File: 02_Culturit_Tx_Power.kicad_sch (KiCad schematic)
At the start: 36 parts, among them U10 TPS22916CNYFPT, U11 SN74AUP2G08RSER, U12 TPS22916CNYFPT, U5 TPS3839A09DBZR, U6 TPS22916CNYFPT, U7 LP5907QMFX-2.8Q1, U8 TPS6282618DMQR, U9 SN74AUP2G08RSER

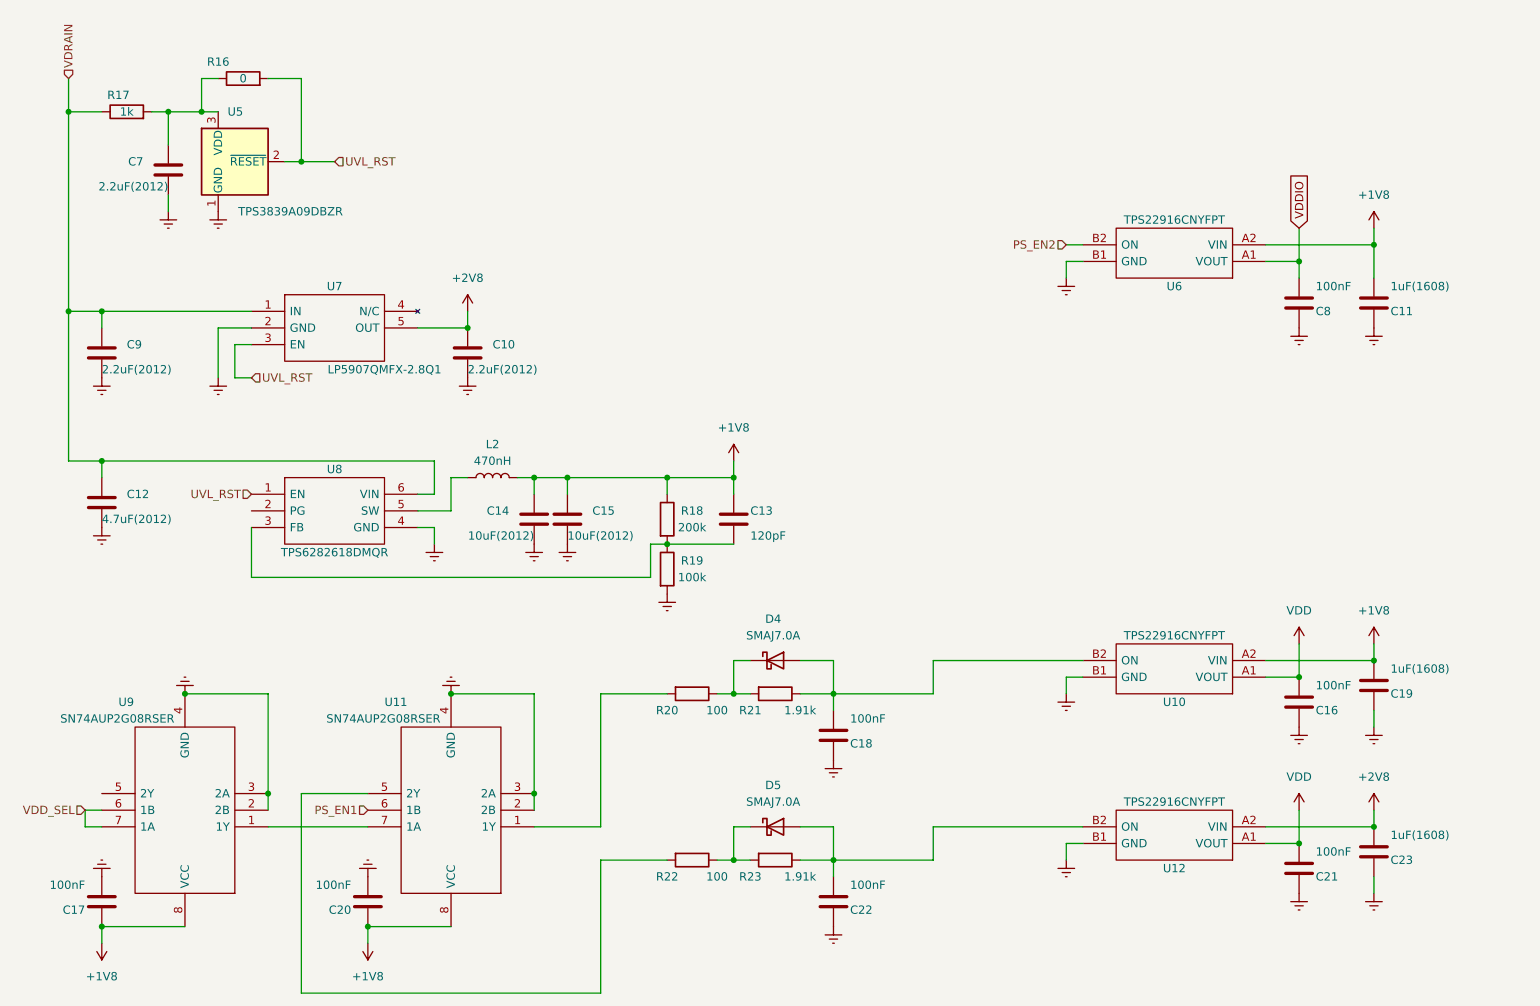
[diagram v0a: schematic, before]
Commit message: 2022-08-26
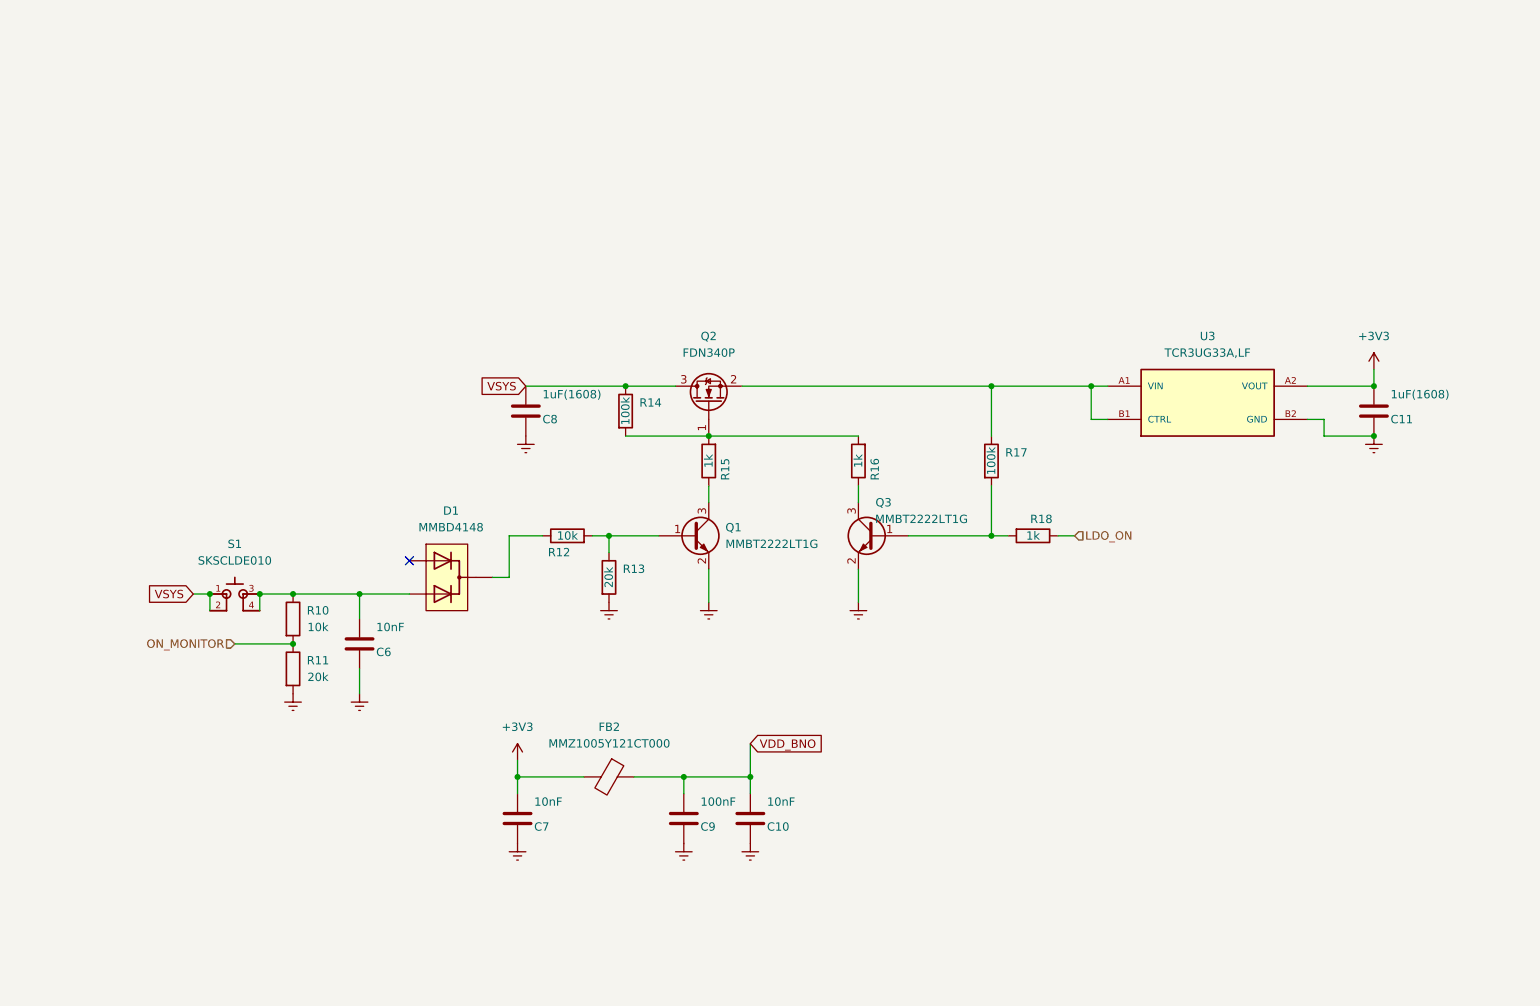
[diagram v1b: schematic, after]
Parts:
- removed C12: 4.7uF(2012), Capacitor_SMD:C_0805_2012Metric, symbol Device:C
- removed C13: 120pF, Capacitor_SMD:C_0402_1005Metric, symbol Device:C
- removed C14, C15: 10uF(2012), Capacitor_SMD:C_0805_2012Metric, symbol Device:C
- removed C16, C17, C18, C20, C21, C22, C8: 100nF, Capacitor_SMD:C_0402_1005Metric, symbol Device:C
- removed C19, C23: 1uF(1608), Capacitor_SMD:C_0603_1608Metric, symbol Device:C
- removed D4, D5: SMAJ7.0A, Diode_SMD:D_SMA, symbol Device:D_Schottky
- removed L2: 470nH, Inductor_SMD:L_0805_2012Metric, symbol Device:L
- removed R20, R22: 100, Resistor_SMD:R_0402_1005Metric, symbol Device:R
- removed R21, R23: 1.91k, Resistor_SMD:R_0402_1005Metric, symbol Device:R
- removed U10, U12, U6: TPS22916CNYFPT, Local_devices:BGA4C40P2X2_78X78X50, symbol TPS22916CNYFPT:TPS22916CNYFPT
- removed U11, U9: SN74AUP2G08RSER, Local_devices:RSE0008A, symbol SN74AUP2G08RSER:SN74AUP2G08RSER
- removed U5: TPS3839A09DBZR, Package_TO_SOT_SMD:SOT-23, symbol Power_Supervisor:TPS3839DBZ
- removed U7: LP5907QMFX-2.8Q1, Local_devices:SOT95P280X145-5N, symbol LP5907QMFX-2.8Q1:LP5907QMFX-2.8Q1
- removed U8: TPS6282618DMQR, Local_devices:TPS6282618DMQR, symbol TPS6282618DMQR:TPS6282618DMQR
- added C11: 1uF(1608), Capacitor_SMD:C_0603_1608Metric, symbol Device:C
- added C6: 10nF, Capacitor_SMD:C_0402_1005Metric, symbol Device:C
- added D1: MMBD4148, Local_devices:SOT23, symbol MMBD4148:MMBD4148
- added FB2: MMZ1005Y121CT000, symbol Device:FerriteBead
- added Q1, Q3: MMBT2222LT1G, Local_devices:SOT23, symbol Device:Q_NPN_BEC
- added Q2: FDN340P, Local_devices:SOT23, symbol Device:Q_NMOS_GSD
- added R10, R12: 10k, Resistor_SMD:R_0402_1005Metric, symbol Device:R
- added R11, R13: 20k, Resistor_SMD:R_0402_1005Metric, symbol Device:R
- added R15: 1k, Resistor_SMD:R_0402_1005Metric, symbol Device:R
- added S1: SKSCLDE010, Local_devices:SKSCLDE010, symbol SKSCLDE010:SKSCLDE010
- added U3: TCR3UG33A,LF, Local_devices:BGA4N35P2X2_64X64X33, symbol TCR3UG33A_LF:TCR3UG33A,LF
- C10, C7: value 2.2uF(2012) -> 10nF; footprint Capacitor_SMD:C_0805_2012Metric -> Capacitor_SMD:C_0402_1005Metric; MPN CC0805KKX7R8BB225 -> CC0402KRX7R9BB103
- C9: value 2.2uF(2012) -> 100nF; footprint Capacitor_SMD:C_0805_2012Metric -> Capacitor_SMD:C_0402_1005Metric; MPN CC0805KKX7R8BB225 -> CC0402KRX7R7BB104
- R16: value 0 -> 1k; MPN 0402WGF0000TCE -> RC0402FR-071KL
- R17: value 1k -> 100k; MPN 0402WGJ0102TCE -> RC0402FR-07100KL
- R18: value 200k -> 1k; MPN RTT022003FTH -> RC0402FR-071KL
- renumbered C11 to C8, R19 to R14
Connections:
- net +2V8 is gone; now on net Earth: C10.2
- net Earth: now also C7.2, C9.2, C11.2, C6.2, Q1.2 (E), Q3.2 (E), R11.2, R13.2, U3.B2 (GND); no longer C10.1, C7.1, C9.1, R14.2
- net at R18.2: now also R17.2, Q3.1 (B); no longer R14.1
- net +1V8 renamed LDO_ON
- net LDO_ON: no longer C8.1
- net UVL_RST: no longer names the net of R16.2
- net UVL_RST: now also R14.2, Q2.1 (G), R15.2
- net VDRAIN: no longer names the net of R17.1
- net VDRAIN: now also Q2.2 (S), U3.A1 (VIN), U3.B1 (CTRL); no longer C9.2
- new net: Q3.3 (C), R16.1
- new net: C6.1, D1.2, R10.1, S1.3, S1.4
- new net: Q1.1 (B), R12.2, R13.1
- new net: Q1.3 (C), R15.1
- new net: D1.3, R12.1
- new net +3V3: C11.1, C7.1, FB2.2, U3.A2 (VOUT)
- new net ON_MONITOR: R10.2, R11.1
- new net VDD_BNO: C10.1, C9.1, FB2.1
- new net VSYS: C8.1, Q2.3 (D), R14.1, S1.1, S1.2
- no-connect marks 0 -> 1
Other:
- moved on the sheet: C8, R14

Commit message: 2022-08-29
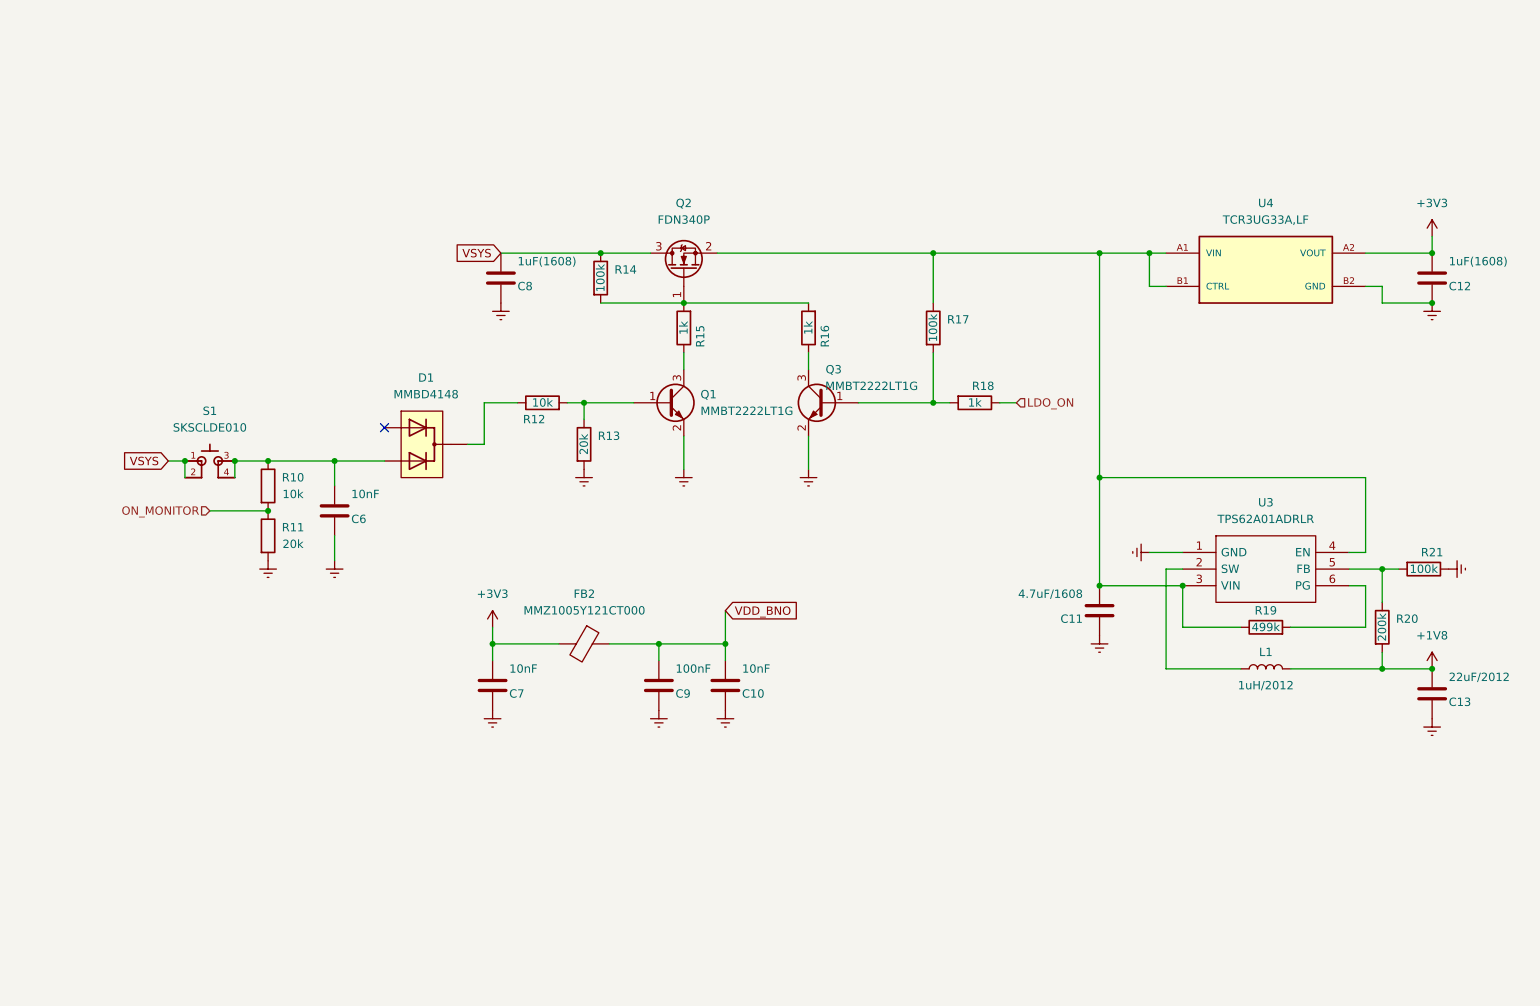
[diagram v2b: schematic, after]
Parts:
- added C11: 4.7uF/1608, Capacitor_SMD:C_0603_1608Metric, symbol Device:C
- added C13: 22uF/2012, Capacitor_SMD:C_0805_2012Metric, symbol Device:C
- added L1: 1uH/2012, Inductor_SMD:L_0805_2012Metric, symbol Device:L
- added R19: 499k, Resistor_SMD:R_0402_1005Metric, symbol Device:R
- added R20: 200k, Resistor_SMD:R_0402_1005Metric, symbol Device:R
- added R21: 100k, Resistor_SMD:R_0402_1005Metric, symbol Device:R
- added U3: TPS62A01ADRLR, Local_devices:SOTFL50P160X60-6N, symbol TPS62A01ADRLR:TPS62A01ADRLR
- renumbered C11 to C12, U3 to U4
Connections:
- net Earth: now also C11.2, C13.2, R21.1, U3.1 (GND)
- net at Q2.2 (S), R17.1, U4.A1 (VIN)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: now also C11.1, R19.1, U3.3 (VIN), U3.4 (EN)
- new net: L1.1, U3.2 (SW)
- new net: R20.1, R21.2, U3.5 (FB)
- new net: R19.2, U3.6 (PG)
- new net +1V8: C13.1, L1.2, R20.2
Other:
- moved on the sheet: C10, C12, C6, C7, C8, C9, D1, FB2, Q1, Q2, Q3, R10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
